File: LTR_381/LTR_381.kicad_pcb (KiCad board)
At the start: 2 copper layers, 25.4 x 17.8 mm, 26 parts, among them J1 Conn_01x06, J2 Conn_01x04, J3 Conn_01x06, J4 Conn_01x04, Q1 BSS138DW, Q2 BSS138DW, U1 AP2127K-3.3

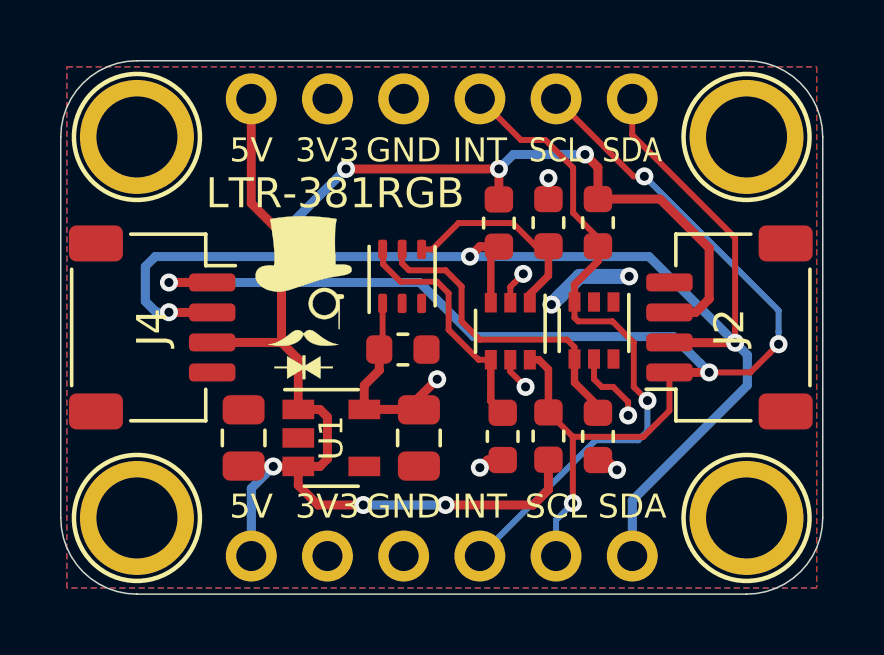
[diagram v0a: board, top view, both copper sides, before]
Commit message: Auto stash before revert of "Board Revision"
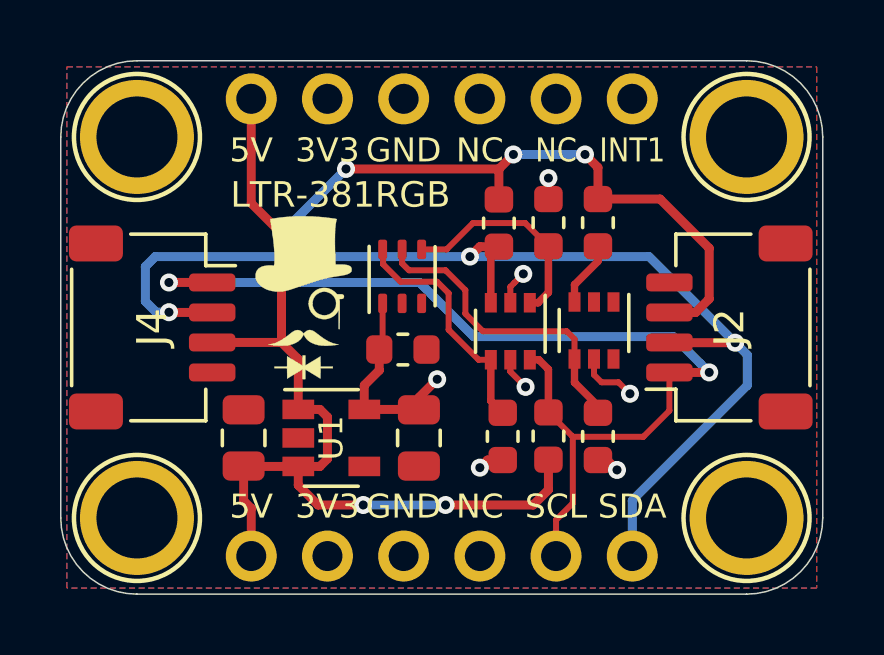
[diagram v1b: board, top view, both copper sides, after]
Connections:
- J1 pad 4: INT_5V -> Net-(J1-Pad4)
- J3 pad 4: INT_5V -> Net-(J3-Pad4)
- J3 pad 5: SCL_5V -> Net-(J3-Pad5)
- J3 pad 6: SDA_5V -> INT1
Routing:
- net INT_5V: track 22.5 -> 2.18 mm, vias 1 -> 0
- net SCL_5V: track 48.6 -> 34.4 mm, vias 5 -> 2
- net SDA_5V: track 48.2 -> 38.7 mm
- net GND: track 2.98 -> 0.00 mm, vias 2 -> 0
- net 3V3: track 14.1 -> 13.5 mm
- net 5V: track 53.9 -> 53.7 mm, vias 7 -> 6
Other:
- board text added: "INT1"
- board text added: "NC"
- board text removed: "INT"
